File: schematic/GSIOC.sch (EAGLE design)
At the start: 39 parts, among them Q1 IRLML5203, X2 PN61729-S, X3 22-23-2081, X6 22-23-2091

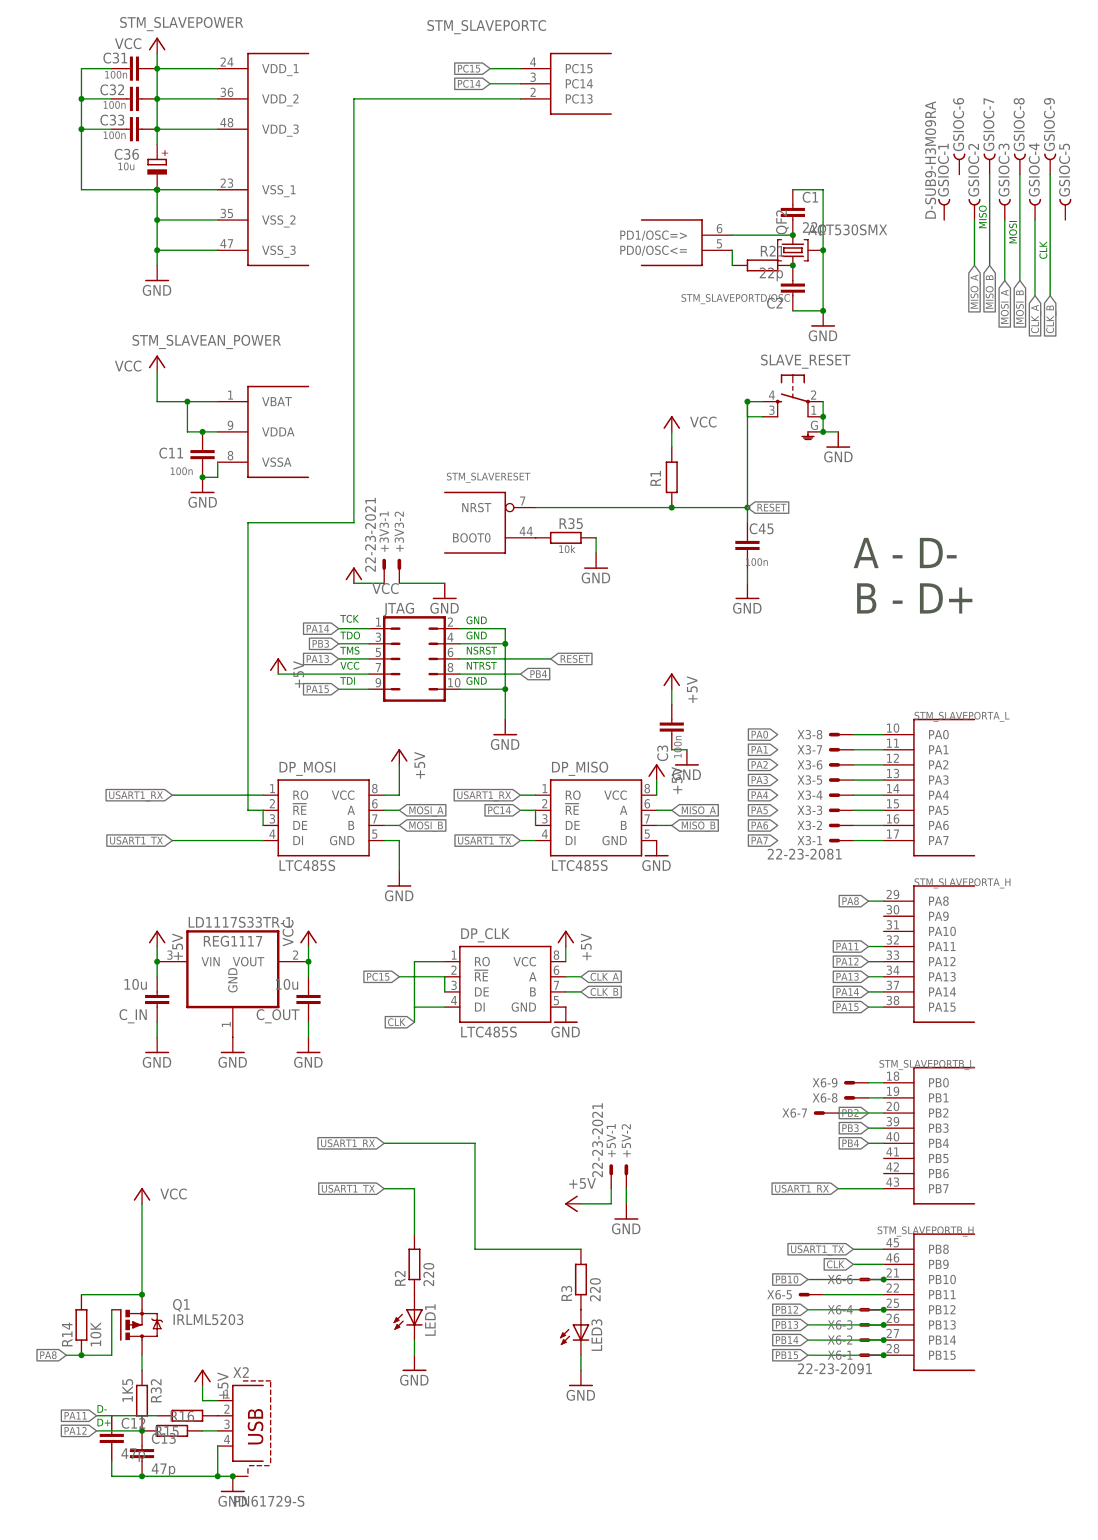
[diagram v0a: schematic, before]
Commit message: cd /home/dekar/eagle/peptidatorV0.51
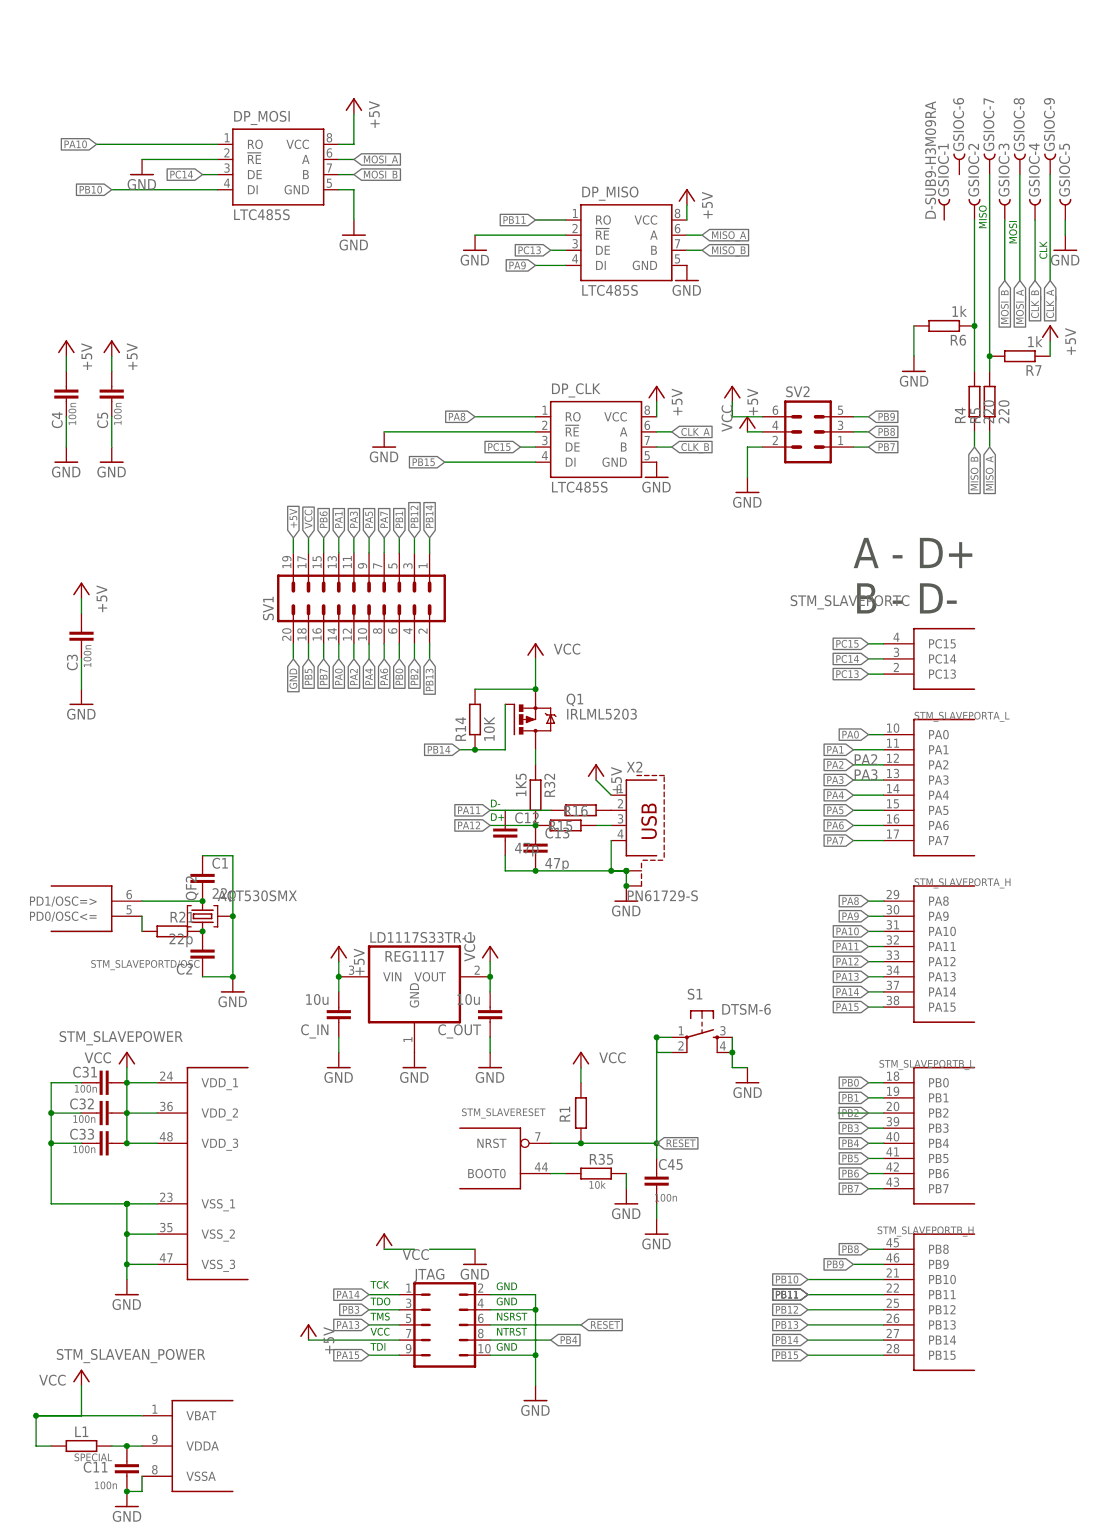
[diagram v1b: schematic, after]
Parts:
- removed +3V3, +5V: 22-23-2021, con-molex:22-23-2021
- removed C36: 10u, resistor:CPOL-EUSMCA
- removed LED1, LED3: (no value), led:LEDSMT1206
- removed R2, R3: 220, resistor:R-EU_M0805
- removed SLAVE_RESET: 10-XXG, switch-omron:10-XXG
- removed X3: 22-23-2081, con-molex:22-23-2081
- removed X6: 22-23-2091, con-molex:22-23-2091
- added C4, C5: 100n, rcl:C-EUC0805K
- added L1: SPECIAL, resistor:R-EU_M0805
- added R4, R5: 220, resistor:R-EU_M0805
- added R6, R7: 1k, resistor:R-EU_M0805
- added S1: DTSM-6, switch-tact:DTSM-6
- added SV1: (no value), con-harting-ml:ML20L
- added SV2: (no value), con-ml:ML6L
- C12, C13, C45: device resistor:C-EUC0805 -> rcl:C-EUC0805K
- C_IN, C_OUT: device rcl:C-EUC1206K -> rcl:C-EUC0805K
- QF2: device crystal:ACT530SMX -> smdQuartz:ACT530SMX
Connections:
- net N$28 renamed OSC<=
- removed net CLK: DP_CLK.DI, DP_CLK.RO, STM_SLAVEPORTB_H.PB9
- removed net N$2: LED3.A, R3.1
- removed net N$34: C1.2, QF2.3, STM_SLAVEPORTD/OSC.PD1/OSC=>
- removed net N$4: STM_SLAVEPORTB_H.PB11, X6-5.S
- removed net USART1_RX: DP_MISO.RO, DP_MOSI.RO, R3.2, STM_SLAVEPORTB_L.PB7
- removed net USART1_TX: DP_MISO.DI, DP_MOSI.DI, R2.2, STM_SLAVEPORTB_H.PB8
- new net N$3: GSIOC-2.F, R4.2, R6.1
- new net N$5: GSIOC-7.F, R5.2, R7.2
- new net OSC=>: C1.2, QF2.2, STM_SLAVEPORTD/OSC.PD1/OSC=>
- new net PA10: DP_MOSI.RO, STM_SLAVEPORTA_H.PA10
- new net PA9: DP_MISO.DI, STM_SLAVEPORTA_H.PA9
- new net PB11: DP_MISO.RO, STM_SLAVEPORTB_H.PB11
- new net PB5: STM_SLAVEPORTB_L.PB5, SV1.18
- new net PB6: STM_SLAVEPORTB_L.PB6, SV1.15
- new net PB7: STM_SLAVEPORTB_L.PB7, SV1.16, SV2.1
- new net PB8: STM_SLAVEPORTB_H.PB8, SV2.3
- new net PB9: STM_SLAVEPORTB_H.PB9, SV2.5
- net +5V: now also C4.1, C5.1, R7.1, SV1.19, SV2.6; no longer +5V-1.S
- net CLK_A: now also GSIOC-9.F; no longer GSIOC-4.F
- net CLK_B: now also GSIOC-4.F; no longer GSIOC-9.F
- net GND: now also C4.2, C5.2, DP_CLK.!RE, DP_MISO.!RE, DP_MOSI.!RE, GSIOC-5.F, QF2.SHLD, R6.2, S1.3, S1.4, SV1.20, SV2.2, X2.S2; no longer +3V3-2.S, +5V-2.S, C36.-, LED1.C, LED3.C, QF2.2, SLAVE_RESET.GND, SLAVE_RESET.P, SLAVE_RESET.P1
- net MISO_A: now also R5.1; no longer GSIOC-2.F
- net MISO_B: now also R4.1; no longer GSIOC-7.F
- net MOSI_A: now also GSIOC-8.F; no longer GSIOC-3.F
- net MOSI_B: now also GSIOC-3.F; no longer GSIOC-8.F
- net N$1: now also C11.1, L1.2, STM_SLAVEAN_POWER.VDDA; no longer LED1.A, R2.1
- net PA0: now also SV1.14; no longer X3-8.S
- net PA1: now also SV1.13; no longer X3-7.S
- net PA2: now also SV1.12; no longer X3-6.S
- net PA3: now also SV1.11; no longer X3-5.S
- net PA4: now also SV1.10; no longer X3-4.S
- net PA5: now also SV1.9; no longer X3-3.S
- net PA6: now also SV1.8; no longer X3-2.S
- net PA7: now also SV1.7; no longer X3-1.S
- net PA8: now also DP_CLK.RO; no longer Q1.G, R14.1
- net PB0: now also SV1.6; no longer X6-9.S
- net PB1: now also SV1.5; no longer X6-8.S
- net PB10: now also DP_MOSI.DI; no longer X6-6.S
- net PB12: now also SV1.3; no longer X6-4.S
- net PB13: now also SV1.2; no longer X6-3.S
- net PB14: now also Q1.G, R14.1, SV1.1; no longer X6-2.S
- net PB15: now also DP_CLK.DI; no longer X6-1.S
- net PB2: now also SV1.4; no longer X6-7.S
- net PC13: now also DP_MISO.DE; no longer DP_MOSI.!RE, DP_MOSI.DE
- net PC14: now also DP_MOSI.DE; no longer DP_MISO.!RE, DP_MISO.DE
- net PC15: no longer DP_CLK.!RE
- net RESET: now also S1.1, S1.2; no longer SLAVE_RESET.S, SLAVE_RESET.S1
- net VCC: now also L1.1, SV1.17, SV2.4; no longer +3V3-1.S, C11.1, C36.+, STM_SLAVEAN_POWER.VDDA
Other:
- note added: "A - D+ B - D-"
- note removed: "A - D- B - D+"
- moved on the sheet: C1, C11, C12, C13, C2, C3, C31, C32, C33, C45, C_IN, C_OUT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
